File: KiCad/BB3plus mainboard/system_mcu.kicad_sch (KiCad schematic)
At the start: 62 parts, among them IC1 SN74HCS02PWR, IC2 M24C32-DFDW6TP, IC3 SN74LVC1G74DCUR, IC4 SN74LVC1G125DCKR, IC5 STM32G071RBT6, IC6 TPS3851H18EDRBR, IC7 SN74HCS02PWR, Q2 2N7002, Y1 FC-135 32.7680KA-K0

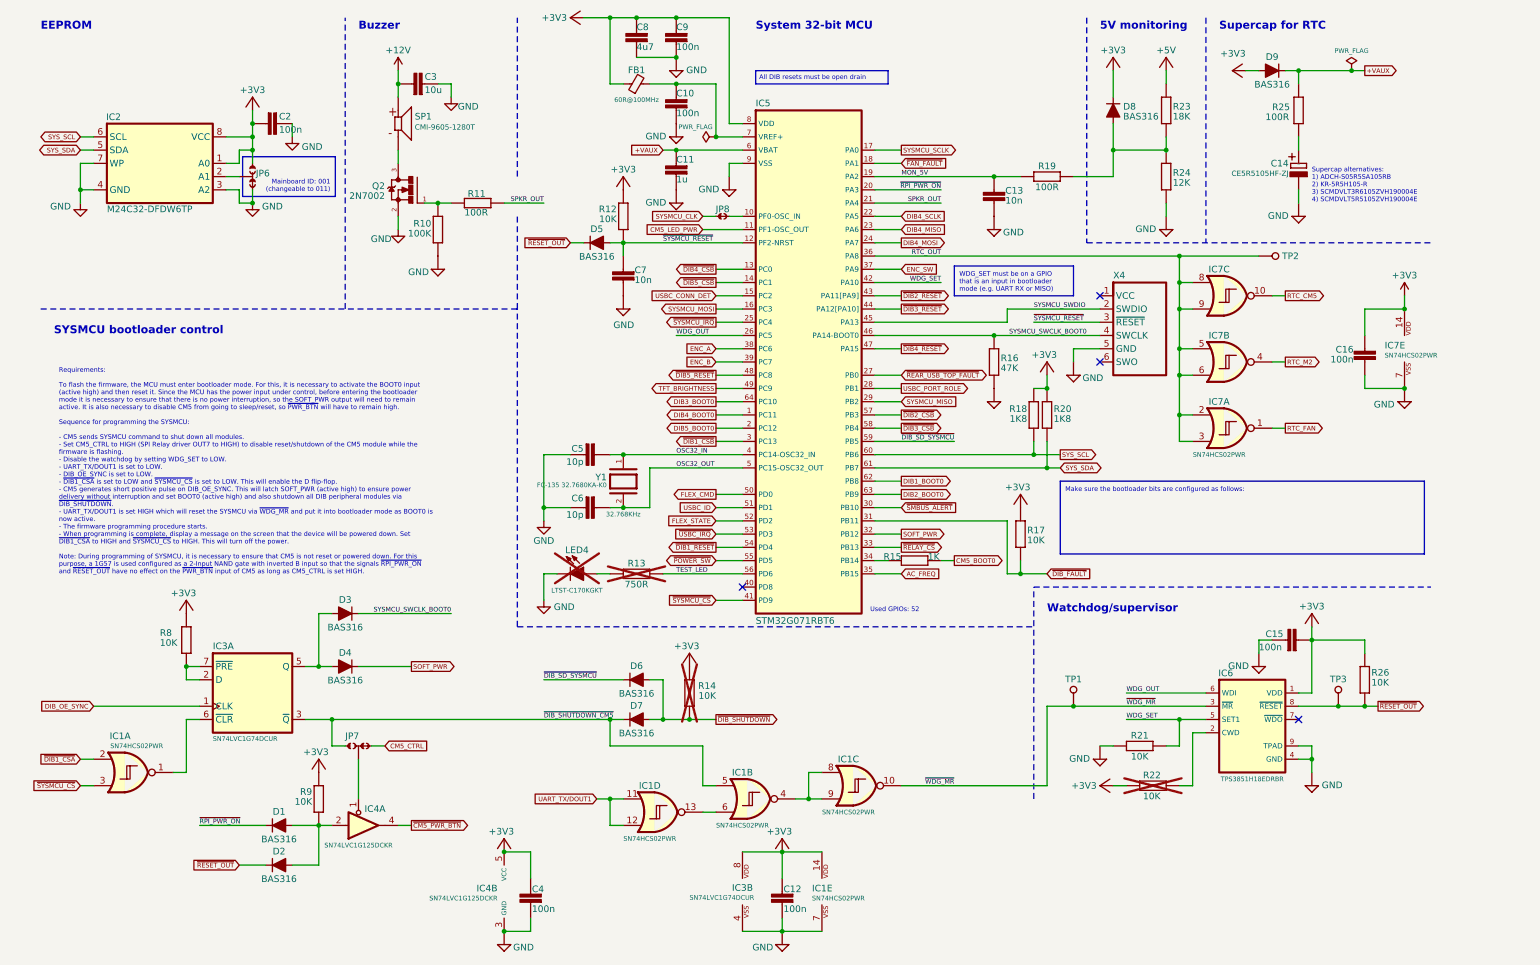
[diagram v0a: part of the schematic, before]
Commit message: #24
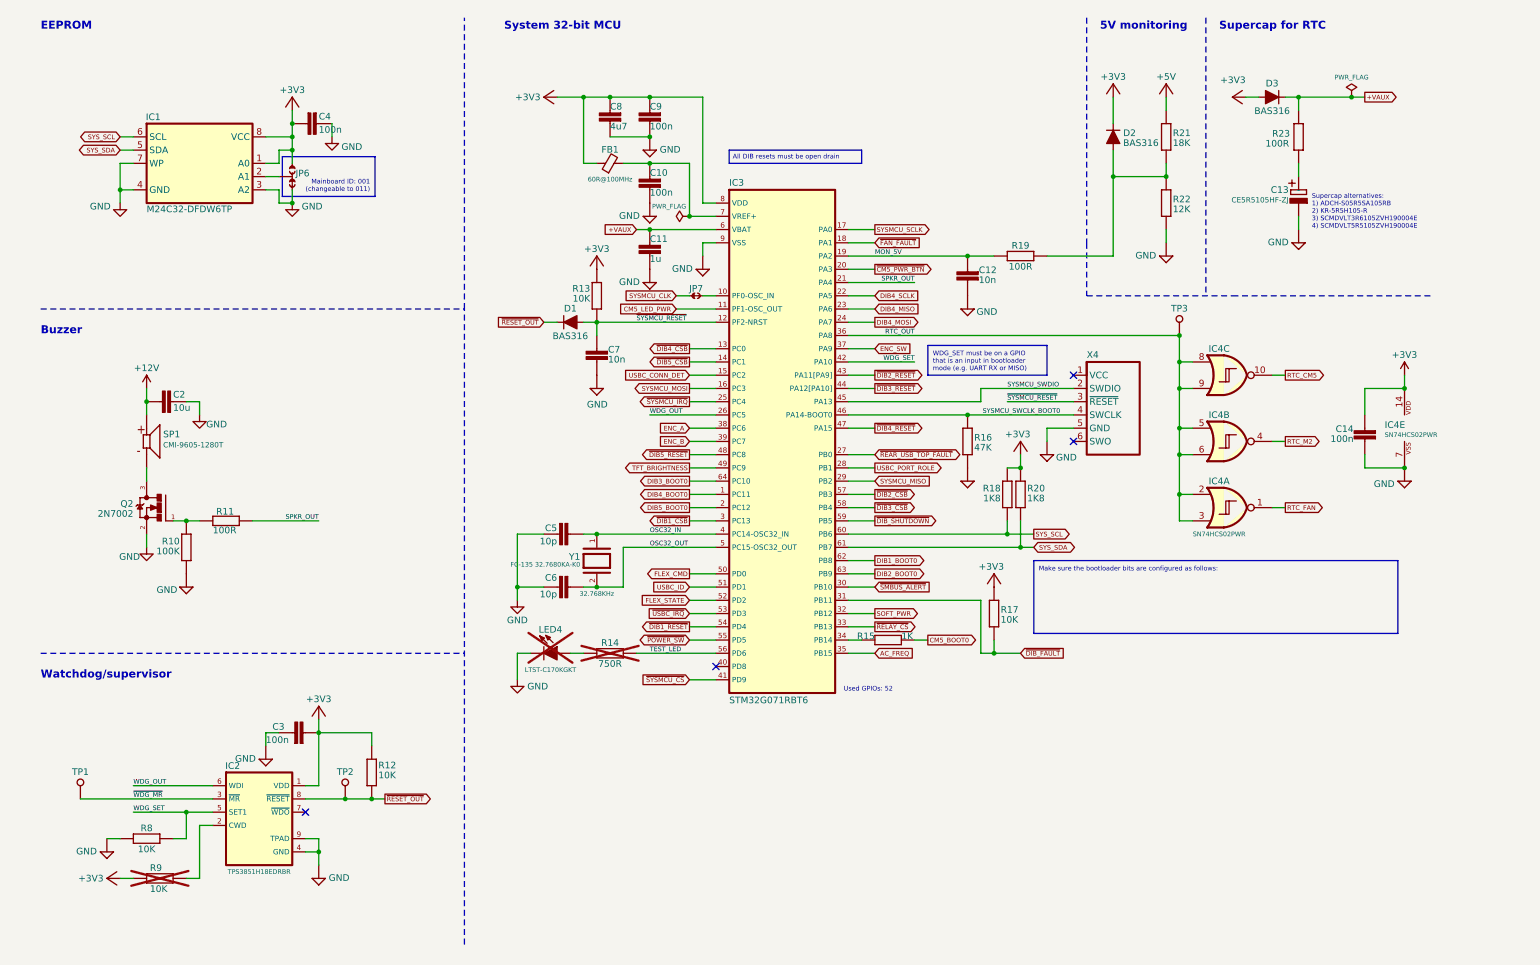
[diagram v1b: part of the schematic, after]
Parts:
- removed C12, C4: 100n, PCM_EEZ_passives:C_0603_1608Metric, symbol PCM_EEZ_passives:C-EU
- removed D1, D2, D3, D4, D6, D7: BAS316, PCM_EEZ_SMD:SOD-323_1P8X1P35_ONS-M, symbol PCM_EEZ_discretes:DIODE
- removed IC1: SN74HCS02PWR, PCM_EEZ_SMD:TSSOP-14, symbol PCM_EEZ_TI:SN74HCS02PWR
- removed IC3: SN74LVC1G74DCUR, PCM_EEZ_SMD:DCU8, symbol PCM_EEZ_TI:SN74LVC1G74DCUR
- removed IC4: SN74LVC1G125DCKR, PCM_EEZ_SMD:SOT65P210X110-5N, symbol PCM_EEZ_TI:SN74LVC1G125DCKR
- removed JP7: (no value), PCM_EEZ_SMD:JP3 shorted (0603), symbol PCM_EEZ_unsorted:JP3 shorted
- removed R14, R8, R9: 10K, PCM_EEZ_passives:R_0603_1608Metric, symbol PCM_EEZ_passives:R-EU
- renumbered C13 to C12, C14 to C13, C16 to C14, C3 to C2, C15 to C3, C2 to C4, D5 to D1, D8 to D2, D9 to D3, IC2 to IC1, IC6 to IC2, IC5 to IC3, IC7 to IC4, JP8 to JP7, R26 to R12, R12 to R13, R13 to R14, R23 to R21, R24 to R22, R25 to R23, R21 to R8, R22 to R9, TP3 to TP2, TP2 to TP3
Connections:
- net ~{DIB_SD_SYSMCU} is gone; now on net ~{DIB_SHUTDOWN}: IC3.59 (PB5)
- net ~{RPI_PWR_ON} is gone; now on net ~{CM5_PWR_BTN}: IC3.20 (PA3)
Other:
- note removed: "SYSMCU bootloader control"
- moved on the sheet: C10, C11, C12, C13, C14, C2, C3, C4, C5, C6, C7, C8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
